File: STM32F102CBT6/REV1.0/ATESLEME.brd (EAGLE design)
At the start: 35.3 x 57.9 mm, 55 parts, among them U1 ADXL345PATRICK, U3 AMS1117-3.3, U4 STM32F102CBT6, Y2 ABM2B-8.000MHZ-10-1-U-T

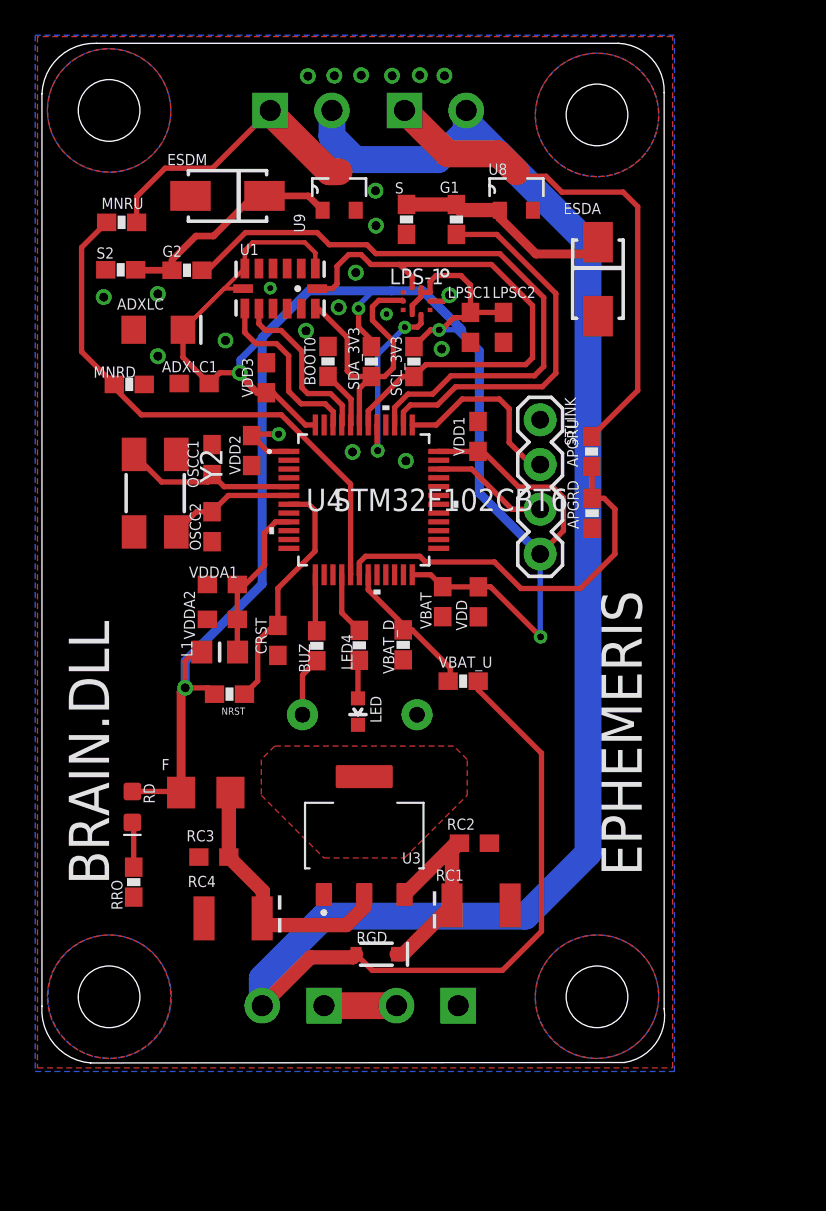
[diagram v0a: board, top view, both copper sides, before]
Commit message: Revision V2.0.0 was released
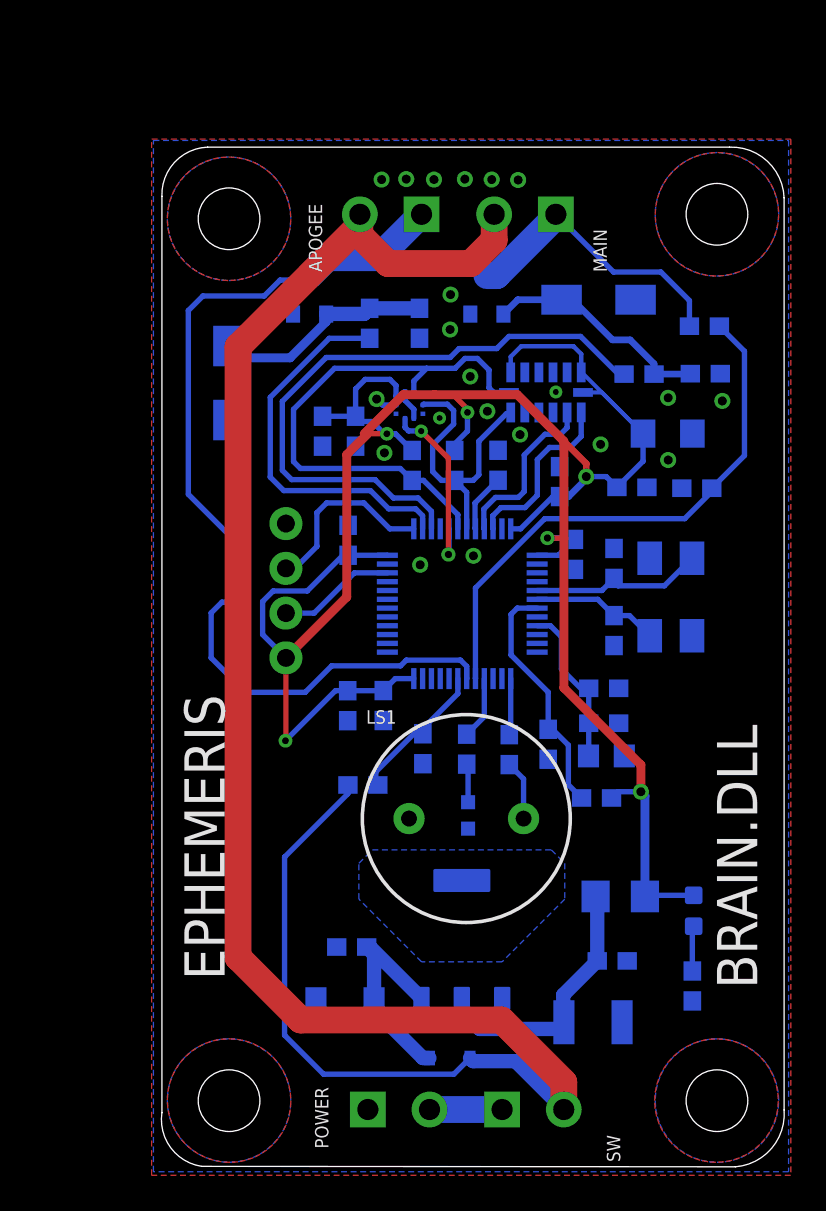
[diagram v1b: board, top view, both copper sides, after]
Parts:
- moved S2 33.7 mm to (31.5, 45.6), flipped to the bottom
- moved MNRU 33.6 mm to (31.4, 48.3), flipped to the bottom
- moved MNRD 32.7 mm to (31.0, 39.1), flipped to the bottom
- moved RD 32.4 mm to (30.8, 15.1), flipped to the bottom
- moved RRO 32.2 mm to (30.7, 10.9), flipped to the bottom
- moved Y2 29.8 mm to (29.5, 32.9), flipped to the bottom
- moved ADXLC 29.5 mm to (29.3, 42.2), flipped to the bottom
- moved G2 26.3 mm to (27.7, 45.6), flipped to the bottom
- moved ADXLC1 25.5 mm to (27.3, 39.2), flipped to the bottom
- moved F 24.2 mm to (26.6, 16.0), flipped to the bottom
- moved OSCC1 23.6 mm to (26.3, 34.8), flipped to the bottom
- moved OSCC2 23.6 mm to (26.3, 31.0), flipped to the bottom
- moved RC3 23.4 mm to (26.2, 12.3), flipped to the bottom
- moved L1 22.7 mm to (25.9, 23.9), flipped to the bottom
- moved VDDA1 22.4 mm to (25.7, 27.8), flipped to the bottom
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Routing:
- added copper zone on layer 16, net HT
- removed copper zone on layer 1, net HT
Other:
- outline, holes or cut-outs redrawn
